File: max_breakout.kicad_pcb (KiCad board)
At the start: 4 copper layers, 51.1 x 25.7 mm, 47 parts, among them J1 USB_B_Micro, J2 Left, J3 AVR-JTAG-10, J4 Right, SW1 User, SW2 Reset, U1 LP2985-5.0, U2 LP2985-3.3, U4 MAX40203AUK+T, U5 74HCT125, U7 EPM7032STC44, U8 74HCT1G04, X1 CTX-636 50mhz

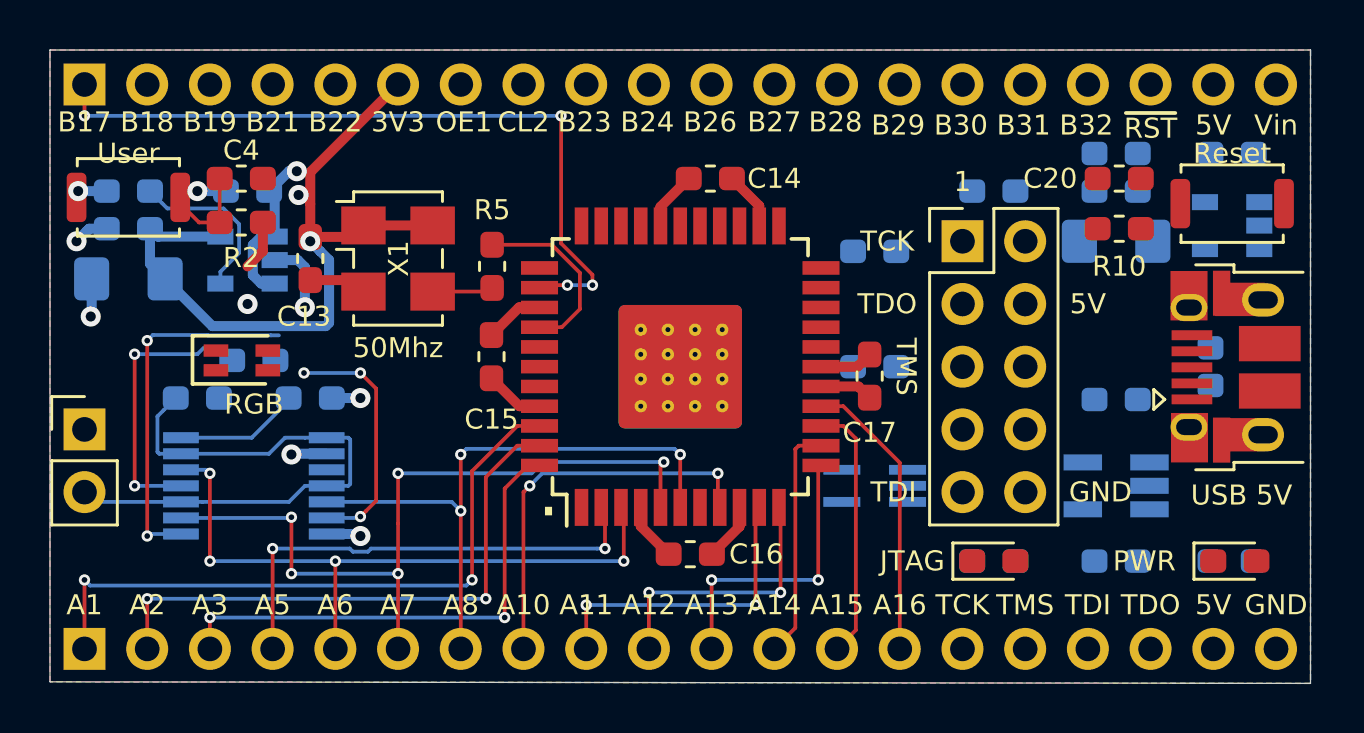
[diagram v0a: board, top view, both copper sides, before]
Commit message: finished routing
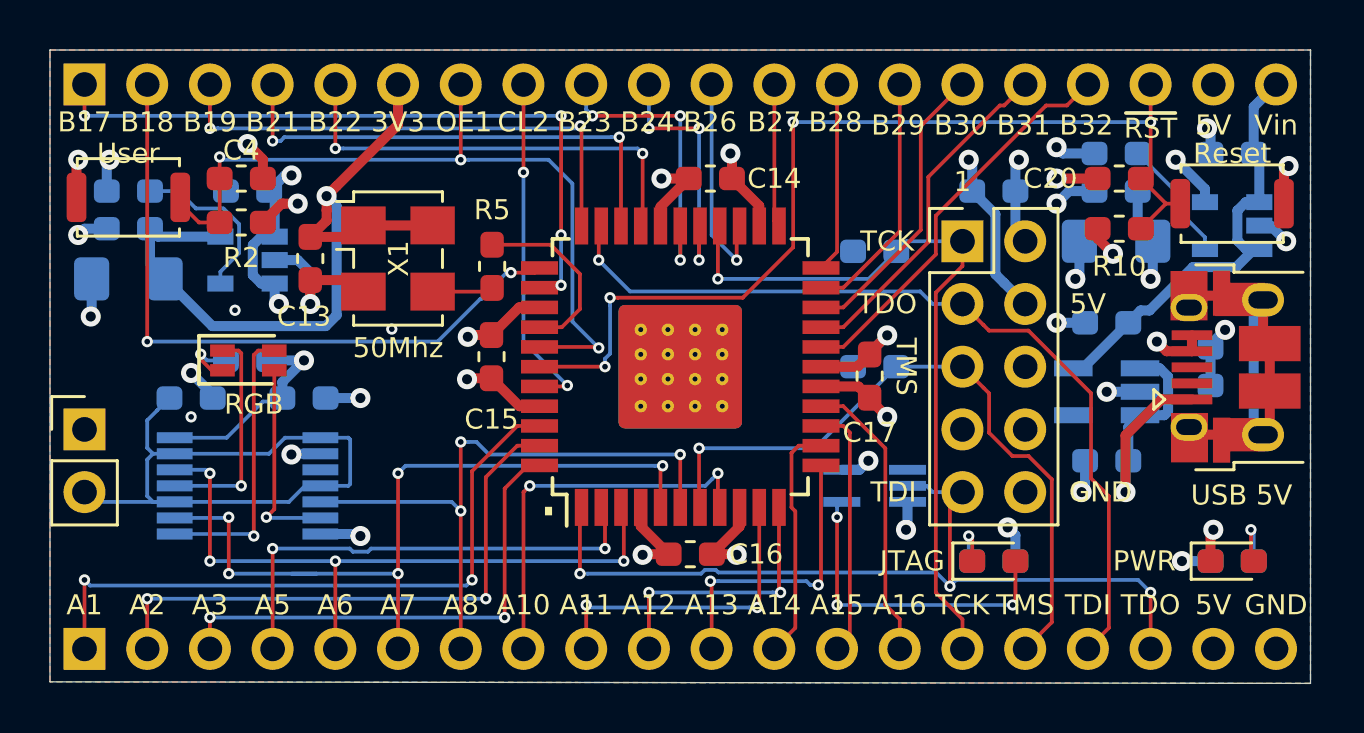
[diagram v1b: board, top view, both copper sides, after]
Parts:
- moved C12 9.66 mm to (167.1, 102.4), turned to 180 degrees
- moved U4 3.83 mm to (167.1, 105.2)
- moved C5 2.51 mm to (167.1, 108.0), turned to 180 degrees
- moved D2 0.26 mm to (132.4, 103.9)
- moved C18 0.25 mm to (134.6, 105.4)
- moved R4 0.25 mm to (132.3, 103.9)
- moved R9 0.25 mm to (130.0, 105.4)
- moved U5 0.25 mm to (132.3, 109.0)
- moved D1 0.11 mm to (172.2, 112.0)
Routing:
- net /~RST: track 0.00 -> 40.8 mm, vias 0 -> 4
- net /TDI: track 0.00 -> 35.1 mm, vias 0 -> 3
- net /TDO: track 0.00 -> 34.6 mm, vias 0 -> 1
- net GND: track 23.9 -> 58.0 mm, vias 9 -> 32
- net /TCK: track 0.00 -> 30.1 mm, vias 0 -> 1
- net /TMS: track 0.00 -> 28.2 mm, vias 0 -> 1
- net /OE1: track 3.69 -> 31.9 mm, vias 0 -> 3
- net /B18: track 0.00 -> 27.6 mm, vias 0 -> 2
- net 5V: track 23.1 -> 50.7 mm, vias 2 -> 15
- net /B19: track 0.00 -> 20.9 mm, vias 0 -> 2
- net /B21: track 0.00 -> 20.0 mm, vias 0 -> 2
- net /B22: track 0.00 -> 18.1 mm, vias 0 -> 2
- net Vin: track 0.00 -> 18.0 mm
- net Net-(C1-Pad1): track 0.00 -> 17.6 mm
- net /B32: track 0.00 -> 16.1 mm
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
